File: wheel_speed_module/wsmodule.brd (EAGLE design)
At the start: 21.3 x 48.2 mm, 19 parts, among them T1 BC849, U1 LTC2875XS

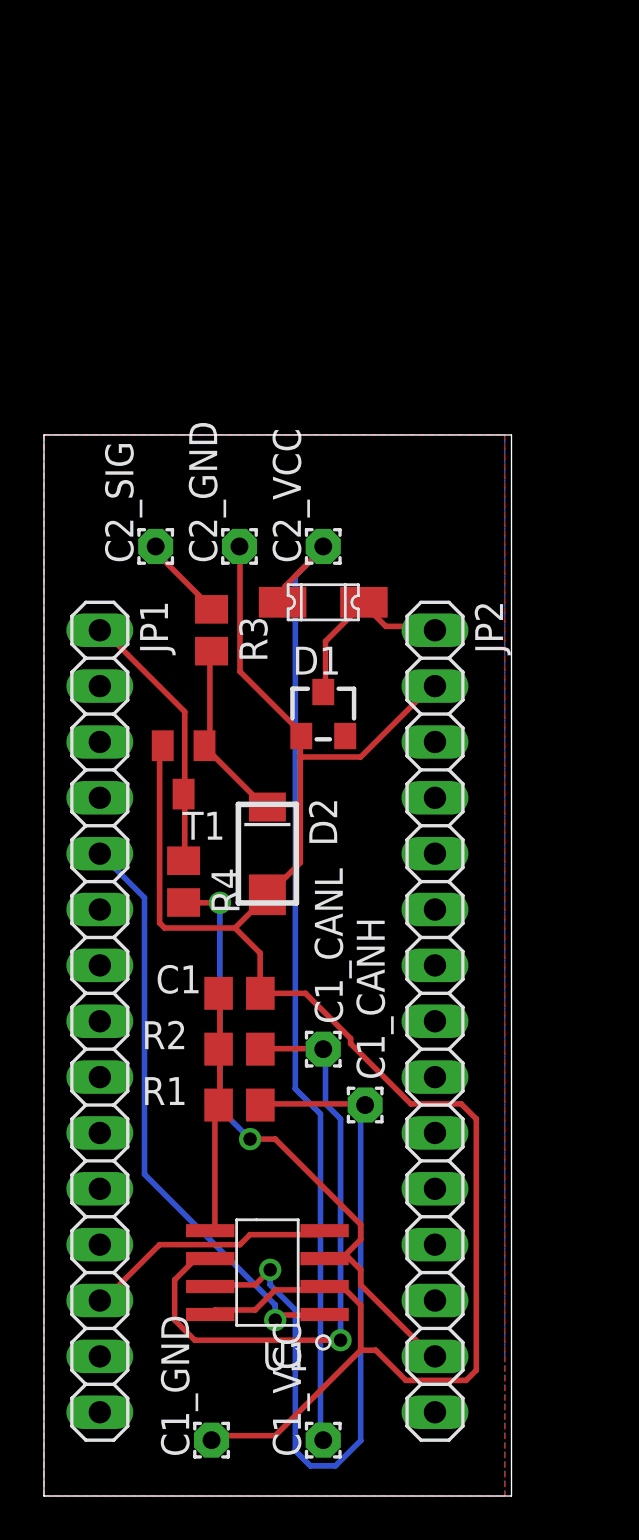
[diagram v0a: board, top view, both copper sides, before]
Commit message: Version 1.1
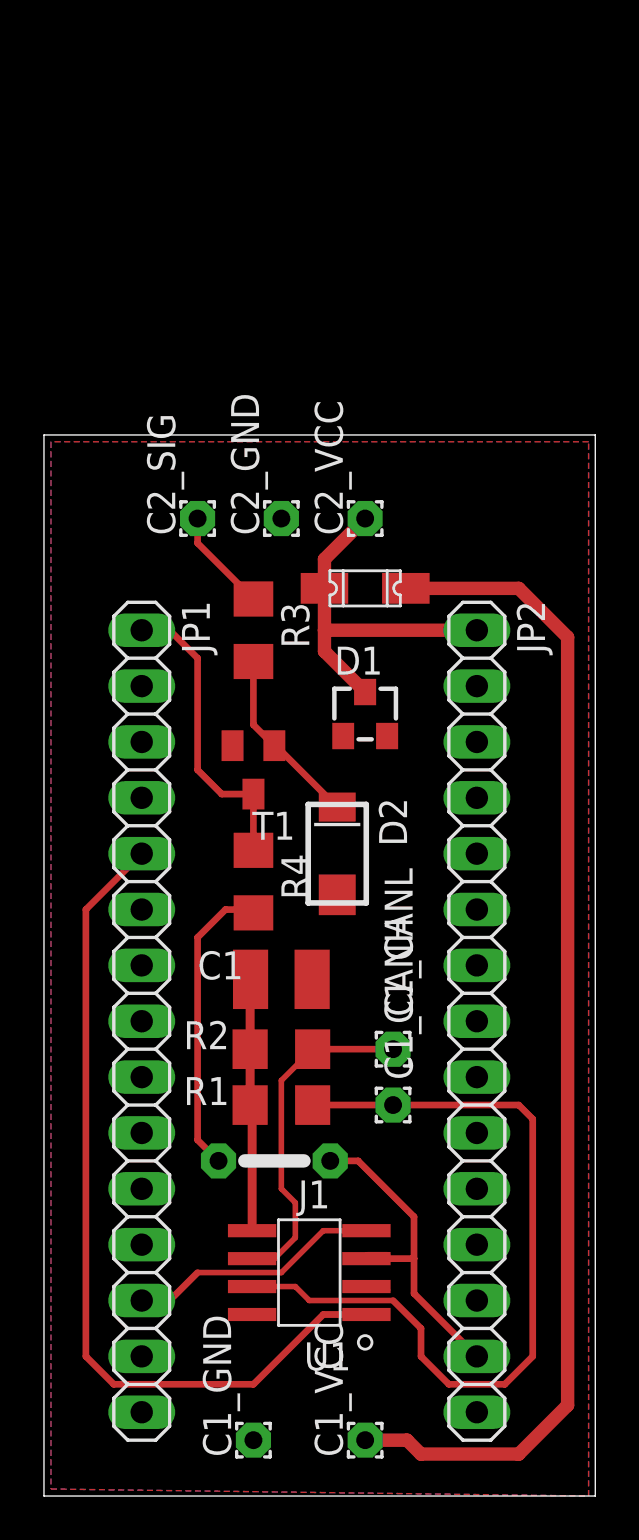
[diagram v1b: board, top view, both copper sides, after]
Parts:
- added J1: J5MM, jumper:05
- C1: value (none) -> 47u; device eagle-ltspice:C0805 -> eagle-ltspice:C1210
- R1, R2, R3, R4: device eagle-ltspice:R0805 -> eagle-ltspice:R1206
- moved C1_CANL 3.18 mm to (15.9, 20.3)
- moved D2 3.18 mm to (13.3, 29.2)
- moved R4 3.18 mm to (9.53, 27.9)
- moved T1 3.18 mm to (9.53, 33.0)
- moved C2_VCC 2.29 mm to (14.6, 44.5)
- moved C2_SIG 2.29 mm to (6.99, 44.5)
- moved C2_GND 2.29 mm to (10.8, 44.5)
- moved F1 2.01 mm to (14.6, 41.3), turned to 0 degrees
- moved C1 2.01 mm to (10.8, 23.5)
- moved C1_VCC 1.91 mm to (14.6, 2.54)
- moved D1 1.91 mm to (14.6, 35.6)
- moved C1_GND 1.91 mm to (9.53, 2.54)
- moved JP1 1.91 mm to (4.45, 21.6)
- moved R3 1.91 mm to (9.53, 39.4)
- moved R1 1.90 mm to (10.8, 17.8)
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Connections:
- new net 3V3R: J1.2, R4.2
- net 3V3: now also J1.1; no longer R4.2
- net GND: now also JP2.12
- net VCC: no longer C2_VCC.1
- net VIN: now also C2_VCC.1
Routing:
- net GND: track 90.4 -> 1.76 mm
- net 3V3: track 29.7 -> 15.3 mm, vias 2 -> 0
- net 3V3R: track 0.00 -> 13.7 mm
- net CANL: track 28.2 -> 15.4 mm, vias 1 -> 0
- net CAN_TX: track 26.9 -> 38.5 mm, vias 1 -> 0
- net VCC: track 45.0 -> 53.6 mm
- net VIN: track 8.68 -> 16.4 mm
- net DIN1: track 12.2 -> 13.7 mm
- net CANH: track 35.6 -> 36.9 mm, vias 1 -> 0
- net HALL1: track 3.93 -> 4.71 mm
- added copper zone on layer 16, net GND
- removed copper zone on layer 16, net VCC
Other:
- board size 21.3 x 48.2 mm -> 25.1 x 48.2 mm

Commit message: Version 1.2
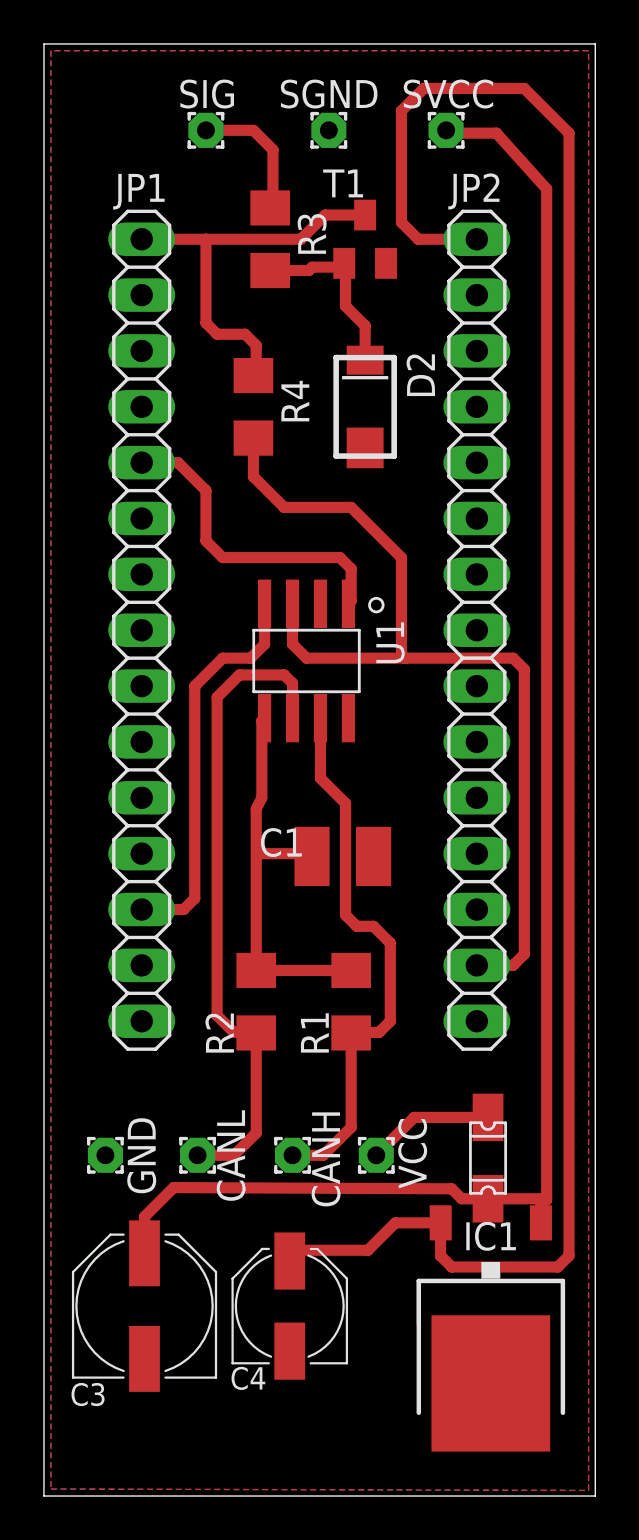
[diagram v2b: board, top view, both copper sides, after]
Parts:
- removed C1_CANH, C1_CANL, C1_GND, C1_VCC, C2_GND, C2_SIG, C2_VCC: WIREPAD1,6/0,8, wirepad:1,6/0,8
- removed D1: BZX84CSMD, diode:TO236
- removed J1: J5MM, jumper:05
- added C3: 100uF, rcl:PANASONIC_D
- added C4: 10uF, rcl:PANASONIC_C
- added CANH, CANL, GND, SGND, SIG, SVCC, VCC: WIREPAD1,6/0,8, wirepad:1,6/0,8
- added IC1: 7805DT, linear:TO252
- moved U1 27.8 mm to (11.9, 38.0), turned to 180 degrees
- moved F1 26.5 mm to (20.2, 15.4), turned to 90 degrees
- moved T1 24.7 mm to (14.6, 57.1), turned to 0 degrees
- moved R4 21.6 mm to (9.53, 49.5)
- moved D2 20.4 mm to (14.6, 49.5)
- moved R3 17.8 mm to (10.3, 57.1)
- moved JP1 17.8 mm to (4.45, 39.4)
- moved JP2 17.8 mm to (19.7, 39.4)
- moved C1 6.25 mm to (13.6, 29.1)
- moved R1 5.67 mm to (14.0, 22.5), turned to 270 degrees
- moved R2 2.44 mm to (9.65, 22.5), turned to 270 degrees
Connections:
- removed net 3V3R: J1.2, R4.2
- new net N$2: C4.+, IC1.2, JP2.1
- net 3V3: now also R4.2; no longer J1.1
- net CANH: now also CANH.1; no longer C1_CANH.1
- net CANL: now also CANL.1; no longer C1_CANL.1
- net GND: now also C3.-, C4.-, GND.1, IC1.3, SGND.1; no longer C1_GND.1, C2_GND.1, D1.A
- net HALL1: now also SIG.1; no longer C2_SIG.1
- net VCC: now also VCC.1; no longer C1_VCC.1
- net VIN: now also C3.+, IC1.1, SVCC.1; no longer C2_VCC.1, D1.C, JP2.1
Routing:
- net N$2: track 0.00 -> 84.3 mm
- net VIN: track 16.4 -> 73.5 mm
- net VCC: track 53.6 -> 5.79 mm
- net 3V3: track 15.3 -> 42.8 mm
- net CAN_TX: track 38.5 -> 14.5 mm
- net CANL: track 15.4 -> 29.8 mm
- net 3V3R: track 13.7 -> 0.00 mm
- net CANH: track 36.9 -> 25.0 mm
- net N$3: track 11.5 -> 18.6 mm
- net CAN_RX: track 11.5 -> 18.1 mm
- net DIN1: track 13.7 -> 18.6 mm
- net GND: track 1.76 -> 0.00 mm
- net HALL1: track 4.71 -> 6.11 mm
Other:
- board size 25.1 x 48.2 mm -> 25.1 x 66 mm
